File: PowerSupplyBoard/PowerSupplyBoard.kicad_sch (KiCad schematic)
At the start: 96 parts, among them J101 BATTERY, J102 I2C, J103 USB_C, J104 PWR, J105 DATA1, Q101 BSH205G2A, Q102 DMP6050SSD, Q103 2N7002H, SW101 SW_SPDT, U101 TPS63070, U102 MCP73834T, U103 NCV33163, U104 CYPD3177-24LQ, U105 CS5173

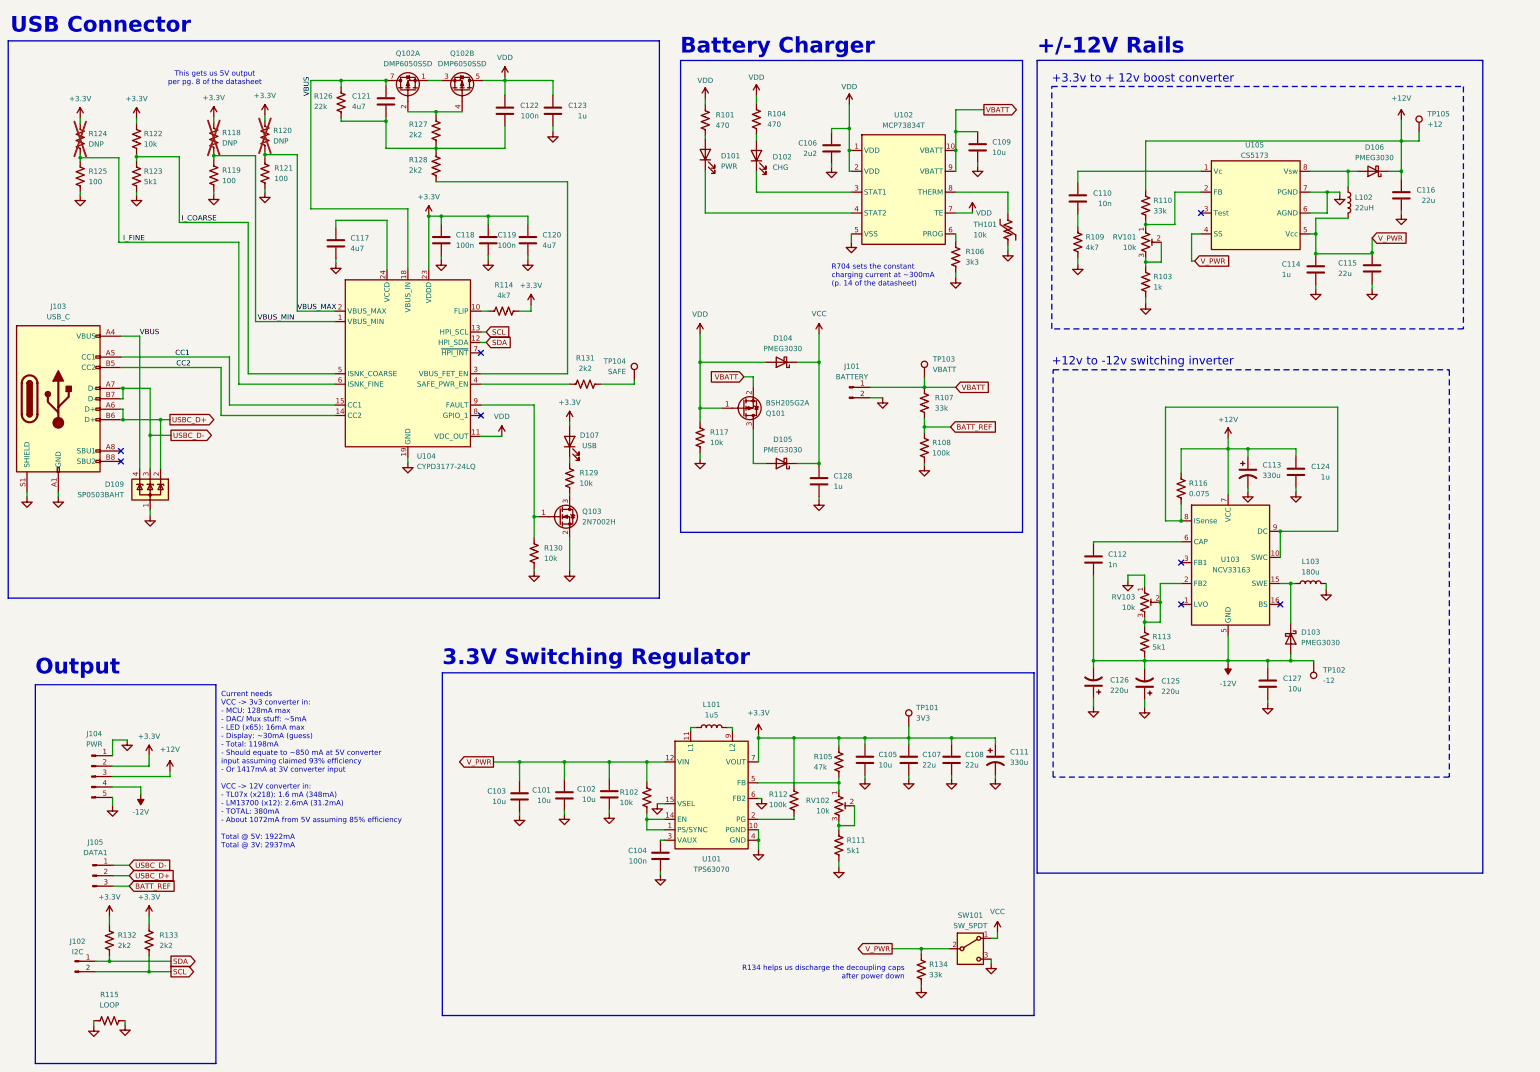
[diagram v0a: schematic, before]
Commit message: psu rev5 layout
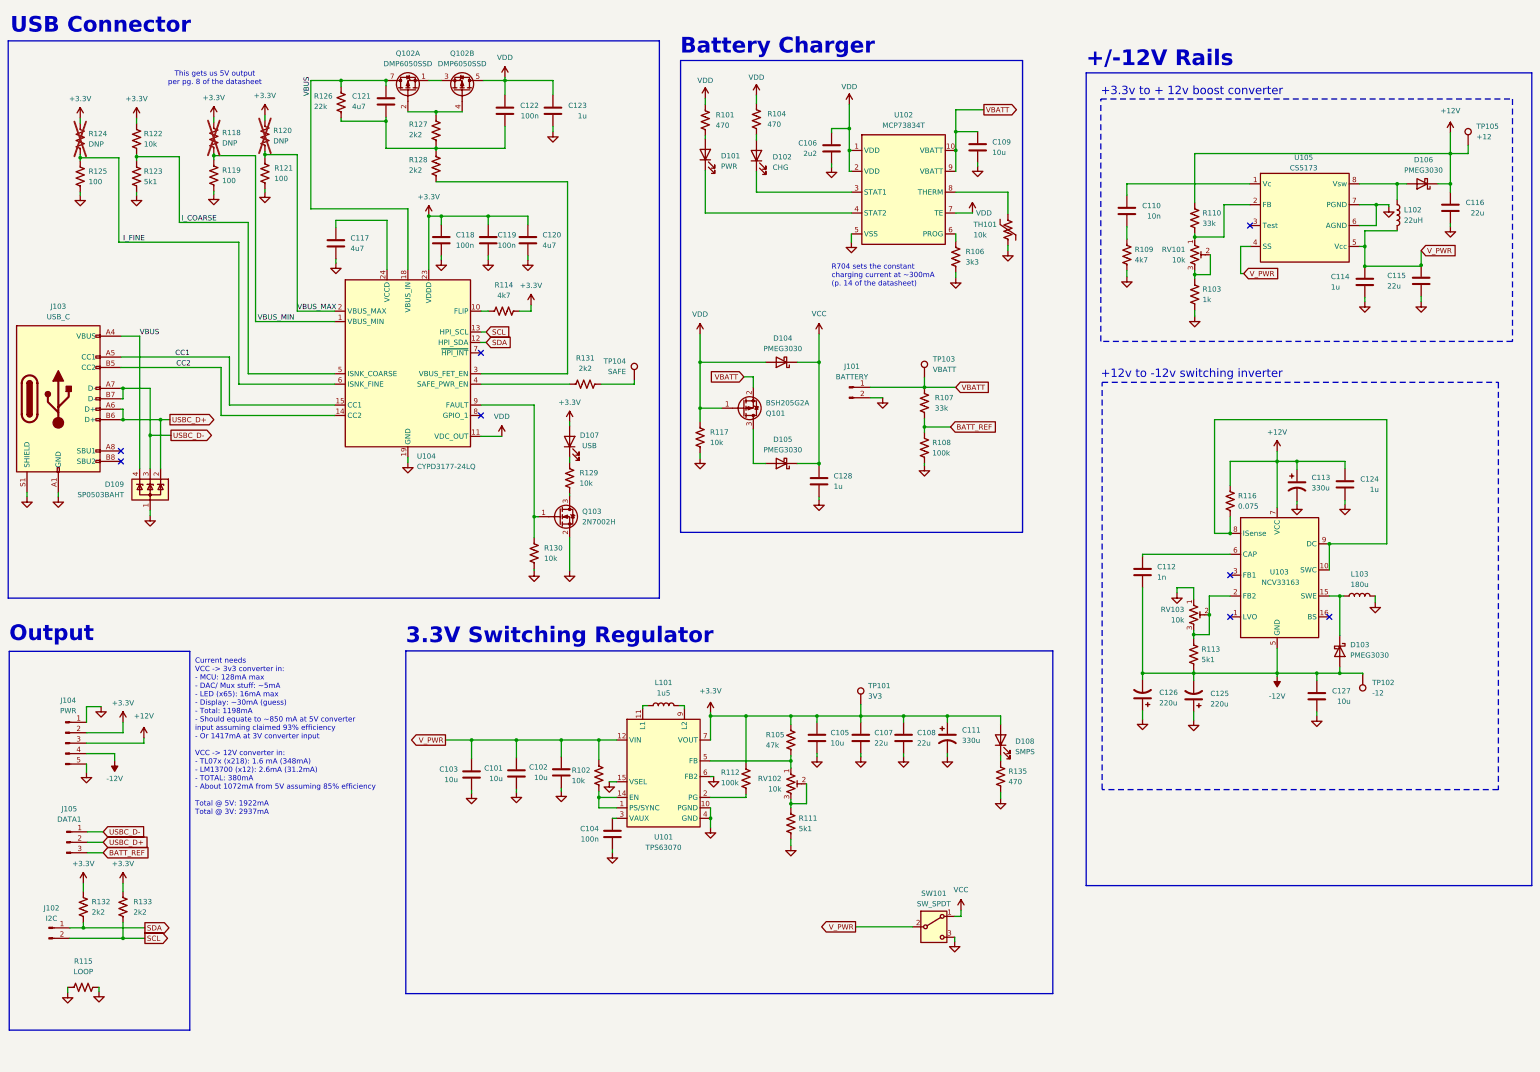
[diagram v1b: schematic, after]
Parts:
- removed R134: 33k, Resistor_SMD:R_0805_2012Metric, symbol Device:R_US
- added D108: SMPS, LED_THT:LED_D3.0mm, symbol Device:LED
- added R135: 470, Resistor_SMD:R_0805_2012Metric, symbol Device:R_US
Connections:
- net +3.3V: now also D108.2 (A)
- net GND: now also R135.2
- new net: D108.1 (K), R135.1
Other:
- note removed: "R134 helps us discharge the decoupling caps after power down"
- moved on the sheet: C101, C102, C103, C104, C105, C107, C108, C110, C111, C112, C113, C114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
